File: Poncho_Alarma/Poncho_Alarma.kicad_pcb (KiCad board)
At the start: 2 copper layers, 41 parts, among them J1 ESP8266, J2 Salidas, J3 Entradas, K1 RELAY_C, K2 RELAY_C, Q1 2N7002, Q2 2N7002, U1 TLP627-4

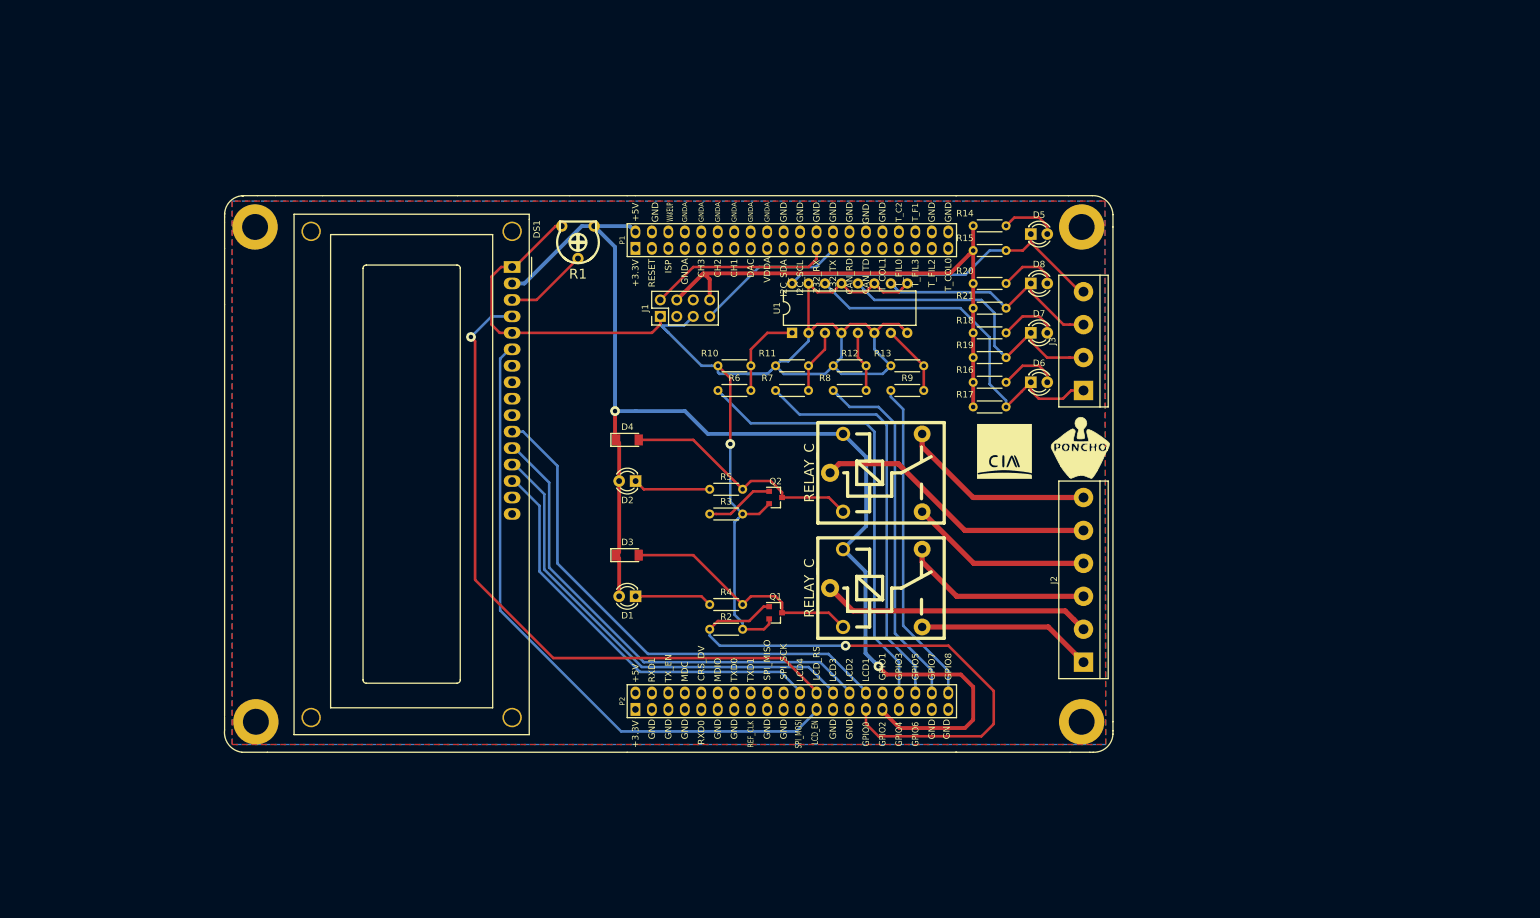
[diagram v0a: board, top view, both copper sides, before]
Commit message: Correcciónes
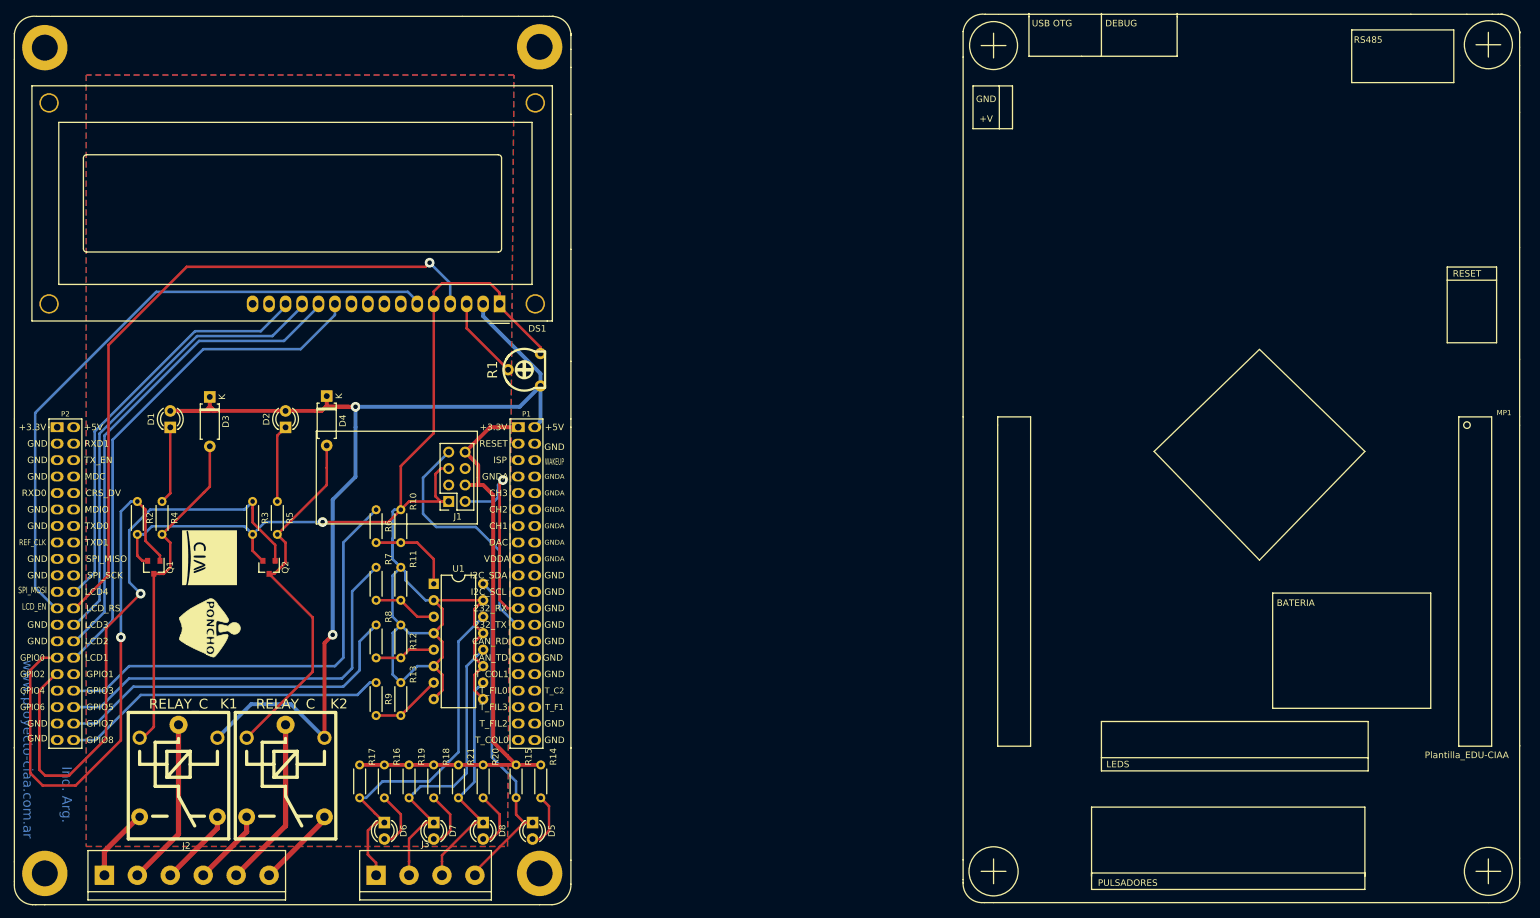
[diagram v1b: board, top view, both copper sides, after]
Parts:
- added MP1: Plantilla_EDU-CIAA, Poncho-PLC:Plantilla_EDU-CIAA, F.Cu at (240.0, 79.0)
- D3, D4: footprint Diode_SMD:D_MiniMELF -> Diode_THT:D_A-405_P7.62mm_Horizontal
- J1: footprint Connector_PinHeader_2.54mm:PinHeader_2x04_P2.54mm_Vertical -> local:ESP-01
- moved J2 154.6 mm to (29.8, 148.4), turned to 0 degrees
- moved G*** 137.1 mm to (46.0, 110.2), turned to 270 degrees
- moved J3 132.3 mm to (71.7, 148.4), turned to 0 degrees
- moved G102 123.7 mm to (46.0, 99.5), turned to 270 degrees
- moved D6 120.7 mm to (73.0, 140.3), turned to 270 degrees
- moved D7 119.1 mm to (80.6, 140.3), turned to 270 degrees
- moved D5 118.9 mm to (95.9, 140.3), turned to 270 degrees
- moved D8 118.5 mm to (88.2, 140.3), turned to 270 degrees
- moved K1 112.5 mm to (41.2, 133.3), turned to 0 degrees
- moved R17 109.6 mm to (69.2, 131.4), turned to 270 degrees
- moved R16 108.3 mm to (73.0, 131.4), turned to 270 degrees
- moved R19 107.3 mm to (76.8, 131.4), turned to 270 degrees
- moved R18 106.6 mm to (80.6, 131.4), turned to 270 degrees
- moved R14 106.6 mm to (97.1, 131.4), turned to 270 degrees
- moved R21 106.2 mm to (84.4, 131.4), turned to 270 degrees
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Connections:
- Q2 pad 1: Net-(Q2-Pad1) -> /Salidas/Out_2
- R3 pad 1: Net-(Q2-Pad1) -> /Salidas/Out_2
- XA1 pad 1: Net-(XA1-Pad1) -> +3V3
- XA1 pad 71: +5V -> /Salidas/Out_2
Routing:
- net /Salidas/Out_2: track 0.00 -> 95.6 mm, vias 0 -> 1
- net +5V: track 196.7 -> 175.9 mm
- net Net-(D4-Pad2): track 37.6 -> 57.3 mm
- net /Salidas/K2_C: track 43.9 -> 26.4 mm
- net /Salidas/K2_NC: track 30.1 -> 12.6 mm
- net /Salidas/K1_NC: track 29.0 -> 12.0 mm
- net /Salidas/K2_NA: track 28.2 -> 11.8 mm
- net /Salidas/K1_C: track 41.7 -> 25.8 mm
- net /Salidas/K1_NA: track 27.1 -> 11.3 mm
- net Net-(J1-Pad7): track 23.5 -> 38.1 mm
- net Net-(D3-Pad2): track 38.1 -> 51.7 mm
- net Net-(Q2-Pad1): track 10.6 -> 0.00 mm
- net +3V3: track 81.5 -> 91.8 mm
- net GND: track 221.3 -> 226.4 mm
- net Net-(J1-Pad2): track 28.4 -> 30.4 mm, vias 0 -> 1
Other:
- board text added: "Ind. Arg."
- board text added: "www.proyecto-ciaa.com.ar"
